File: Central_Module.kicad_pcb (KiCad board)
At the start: 2 copper layers, 32.4 x 31.8 mm, 50 parts, among them J1 USB_B_Micro, J2 SM13B-GHS-TB_LF__SN_, J3 Conn_01x01, J4 Conn_01x01, J5 Conn_01x01, J6 Conn_01x01, J7 Conn_01x01, J8 Conn_01x01, J9 Conn_01x01, Q1 AO3401A, SW1 SW_Push, U1 CH340C, U2 DS3231M, U3 MCP73831-2-MC, U5 ESP32-C3, U7 W25Q32JVSS, U8 AMS1117-3.3, Y1 40MHz

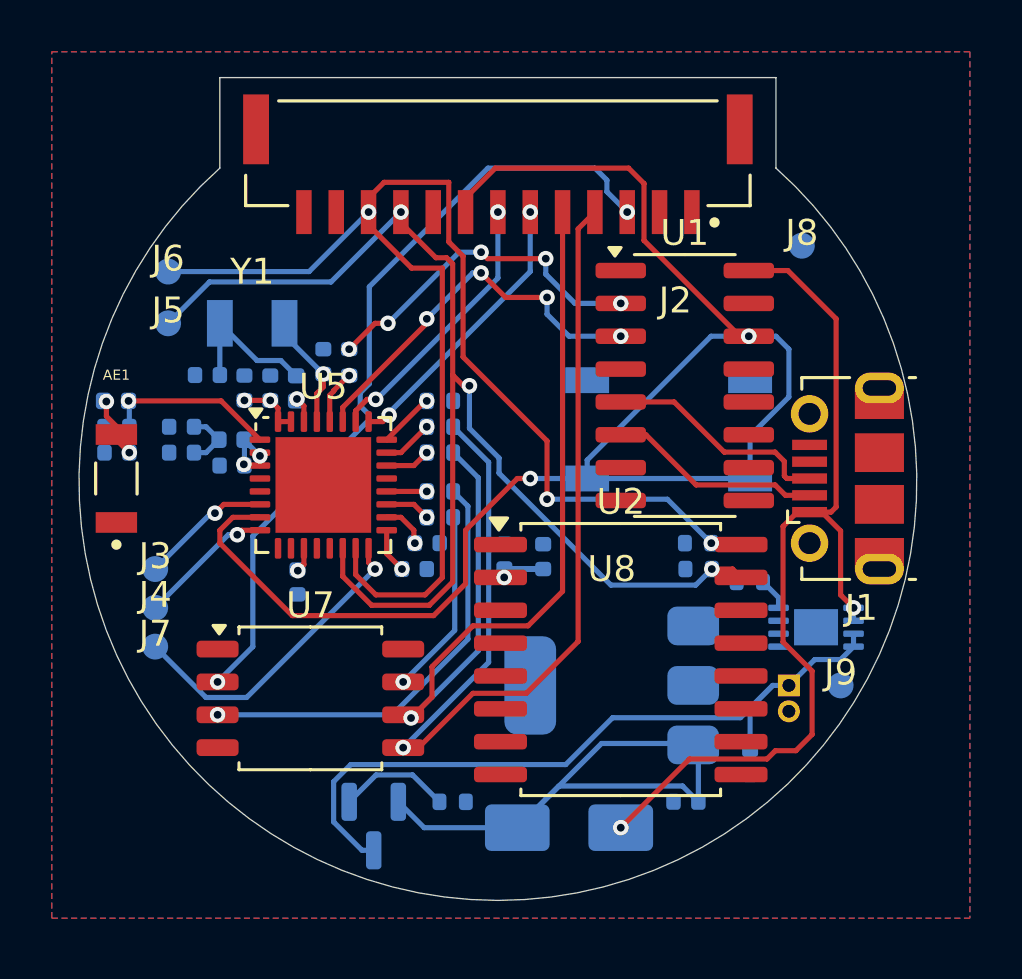
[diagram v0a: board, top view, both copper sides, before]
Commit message: Post DRC Checker
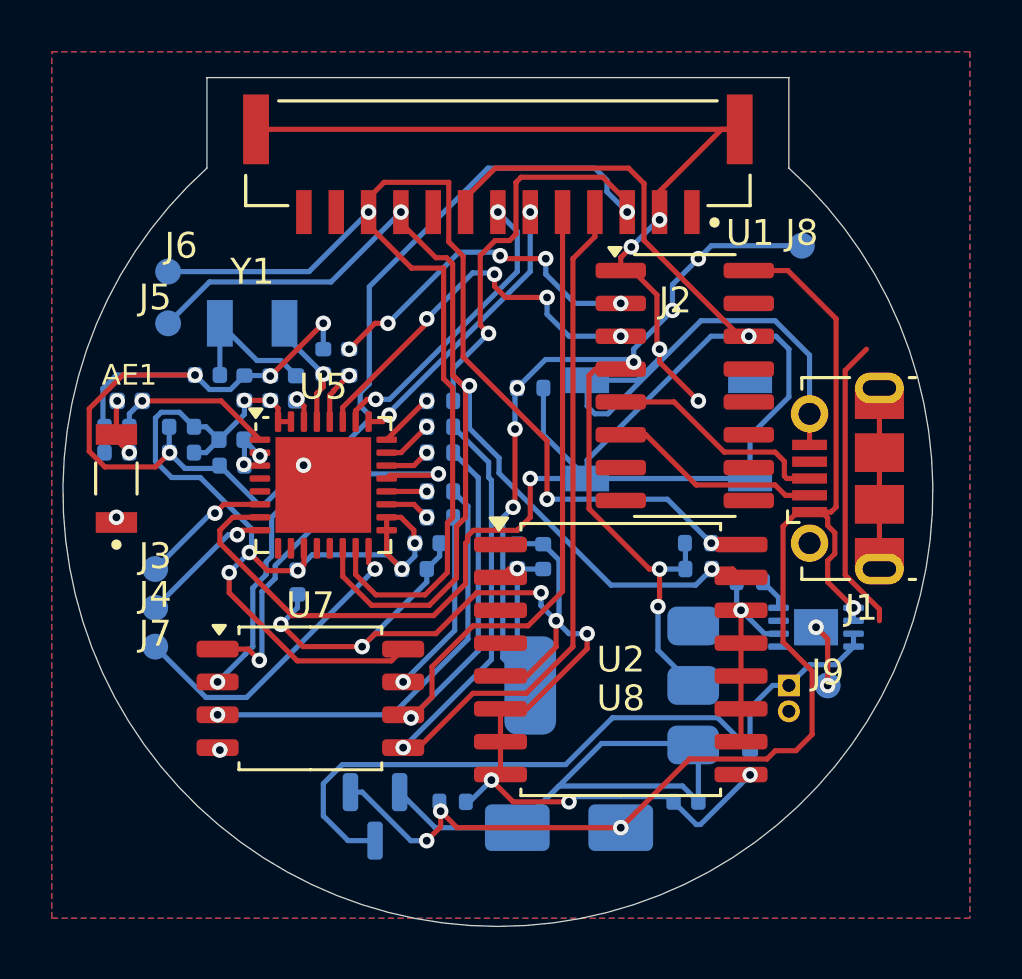
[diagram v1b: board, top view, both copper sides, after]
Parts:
- added R3: 10k, Resistor_SMD:R_0402_1005Metric, B.Cu at (178.0, 96.0)
- moved L1 0.53 mm to (162.5, 96.5)
- moved C4 0.50 mm to (177.5, 102.5)
- moved J9 0.50 mm to (189.5, 107.5)
- moved Q1 0.38 mm to (172.0, 112.6)
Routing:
- net GND: track 0.00 -> 151.9 mm, vias 0 -> 22
- net +3.3V: track 3.50 -> 62.3 mm, vias 1 -> 9
- net TBD: track 9.27 -> 38.7 mm, vias 5 -> 7
- net /CS: track 0.00 -> 15.6 mm, vias 0 -> 2
- net /MISO: track 30.8 -> 46.1 mm, vias 2 -> 3
- net /USB5V: track 40.7 -> 49.3 mm, vias 2 -> 4
- net /RST: track 59.6 -> 64.5 mm
- net /DC: track 10.6 -> 11.5 mm
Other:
- board size 32.4 x 31.8 mm -> 33.6 x 32.8 mm
- board text added: "Angelo Duenas"
